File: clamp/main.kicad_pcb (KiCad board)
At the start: 2 copper layers, 36 parts, among them P1 CONN_01X12, U1 LM741, U2 LM741, U3 LM741, U4 LM741, U5 LM741, U6 LM741

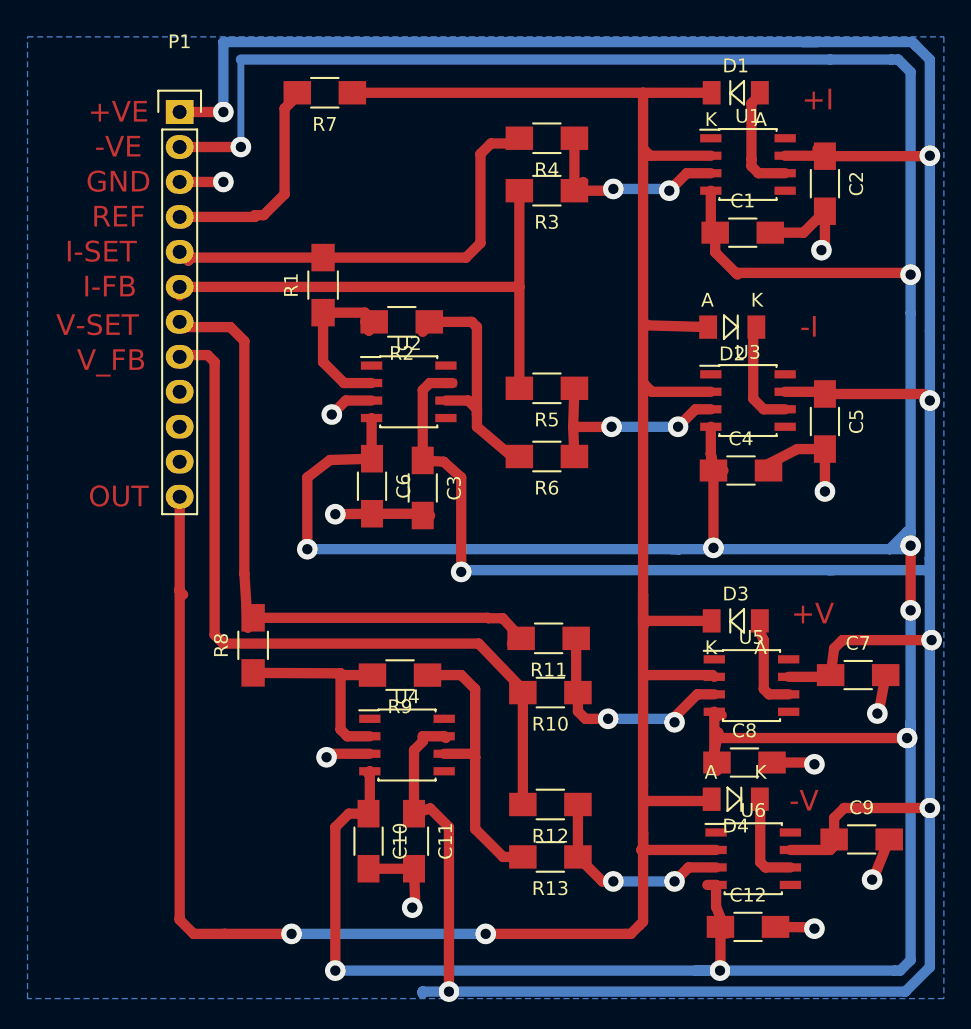
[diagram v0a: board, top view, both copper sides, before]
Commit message: update
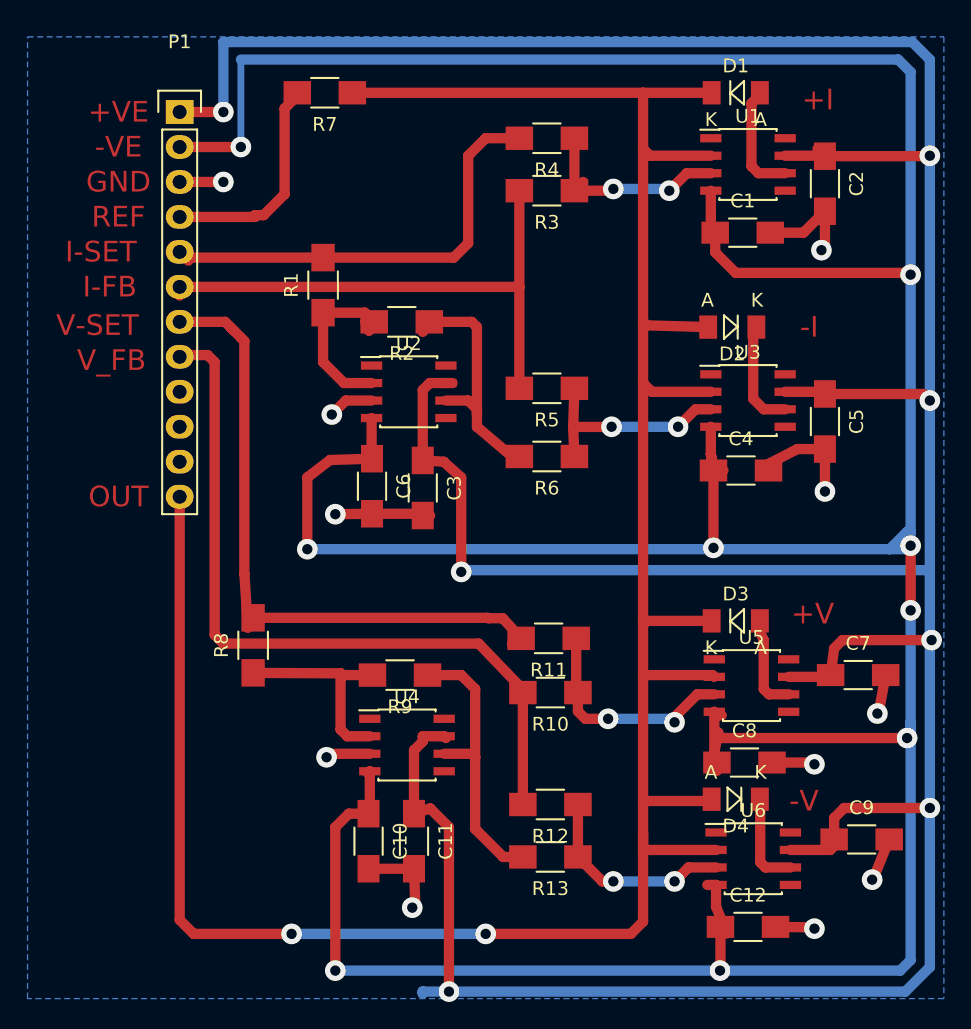
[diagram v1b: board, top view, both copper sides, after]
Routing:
- net -VE: track 307.7 -> 304.4 mm
- net OUT: track 192.5 -> 189.2 mm
- net +VE: track 291.6 -> 288.6 mm
- net I-SET: track 34.3 -> 33.3 mm
- net V-SET: track 48.0 -> 48.9 mm
